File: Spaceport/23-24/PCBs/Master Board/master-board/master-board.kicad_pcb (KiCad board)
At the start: 2 copper layers, 98.7 x 67.9 mm, 10 parts, among them J1 Screw_Terminal_01x02, J2 Conn_01x04_Pin, J3 Conn_01x03_Pin, J4 Conn_01x04_Pin, J5 Conn_01x04_Pin, J6 Conn_01x04_Pin

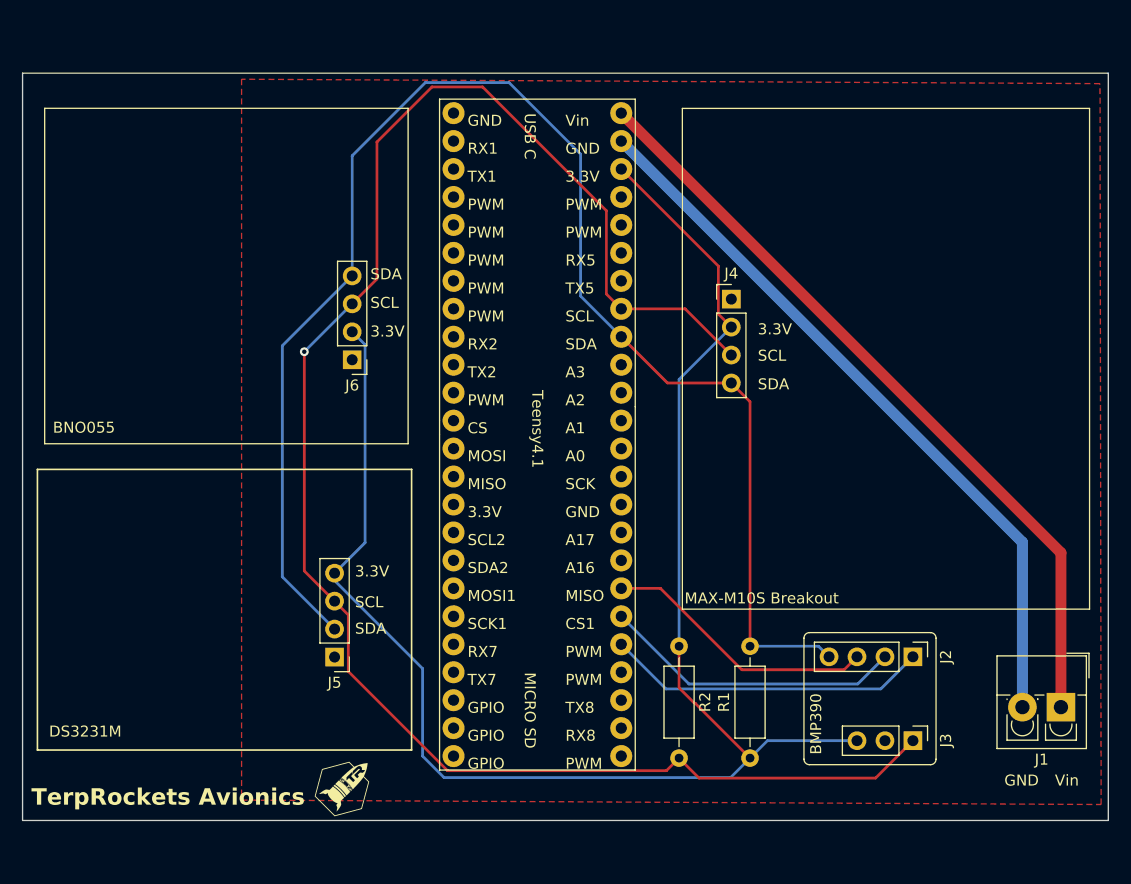
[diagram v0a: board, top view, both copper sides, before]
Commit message: Updated master board
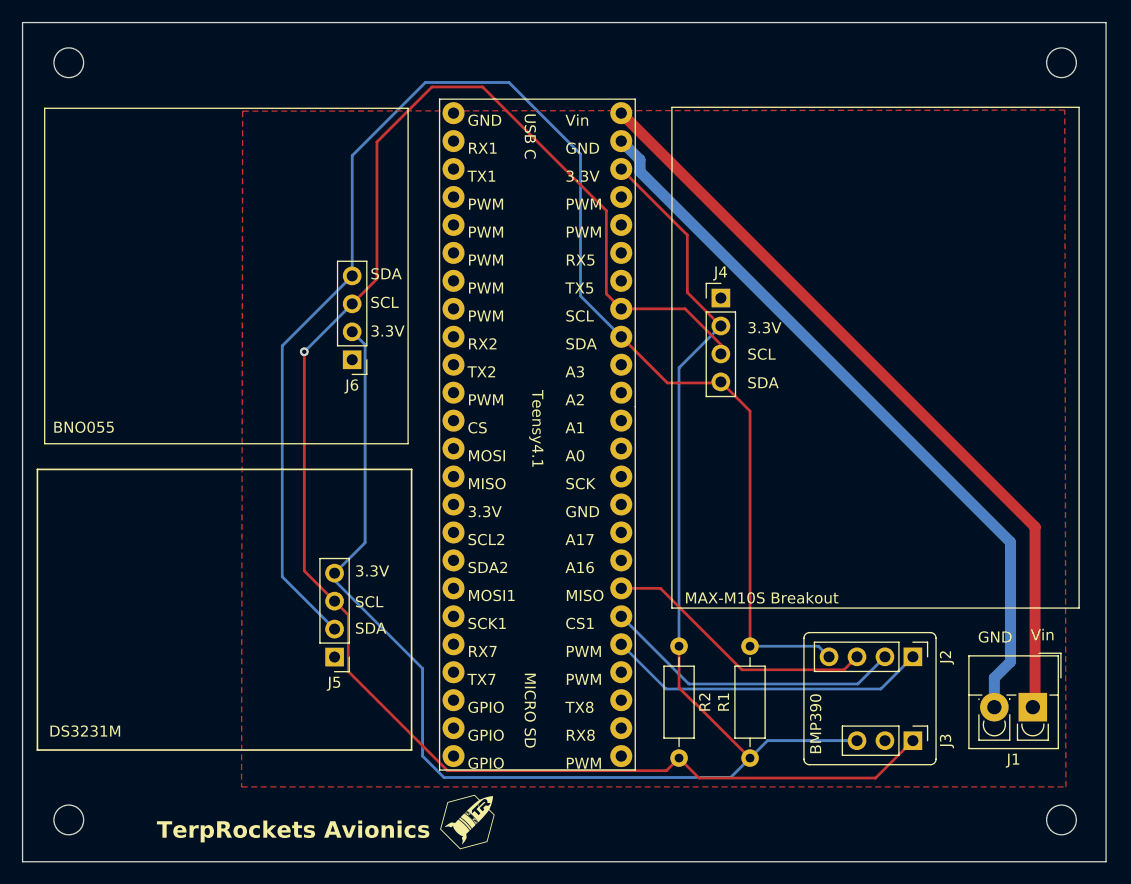
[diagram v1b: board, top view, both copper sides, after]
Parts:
- added H1: MountingHole, MountingHole:MountingHole_2.7mm_M2.5, F.Cu at (183.0, 127.8)
- added H2: MountingHole, MountingHole:MountingHole_2.7mm_M2.5, F.Cu at (183.0, 59.0)
- added H3: MountingHole, MountingHole:MountingHole_2.7mm_M2.5, F.Cu at (92.8, 127.8)
- added H4: MountingHole, MountingHole:MountingHole_2.7mm_M2.5, F.Cu at (92.8, 59.0)
- moved G*** 11.8 mm to (129.0, 128.0)
- moved J1 2.55 mm to (180.4, 117.6)
- moved J4 0.96 mm to (152.1, 80.4)
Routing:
- net Net-(J1-Pin_1): track 70.5 -> 69.6 mm
- net /3.3V: track 147.5 -> 146.7 mm
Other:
- board size 98.7 x 67.9 mm -> 98.5 x 76.2 mm
